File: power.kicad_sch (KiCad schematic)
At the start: 23 parts, among them J11 Conn_01x02_Socket, Q1 IPD068P03L3, U17 CJ9340, U30 ADS1110, U31 LMR51420YDDCR

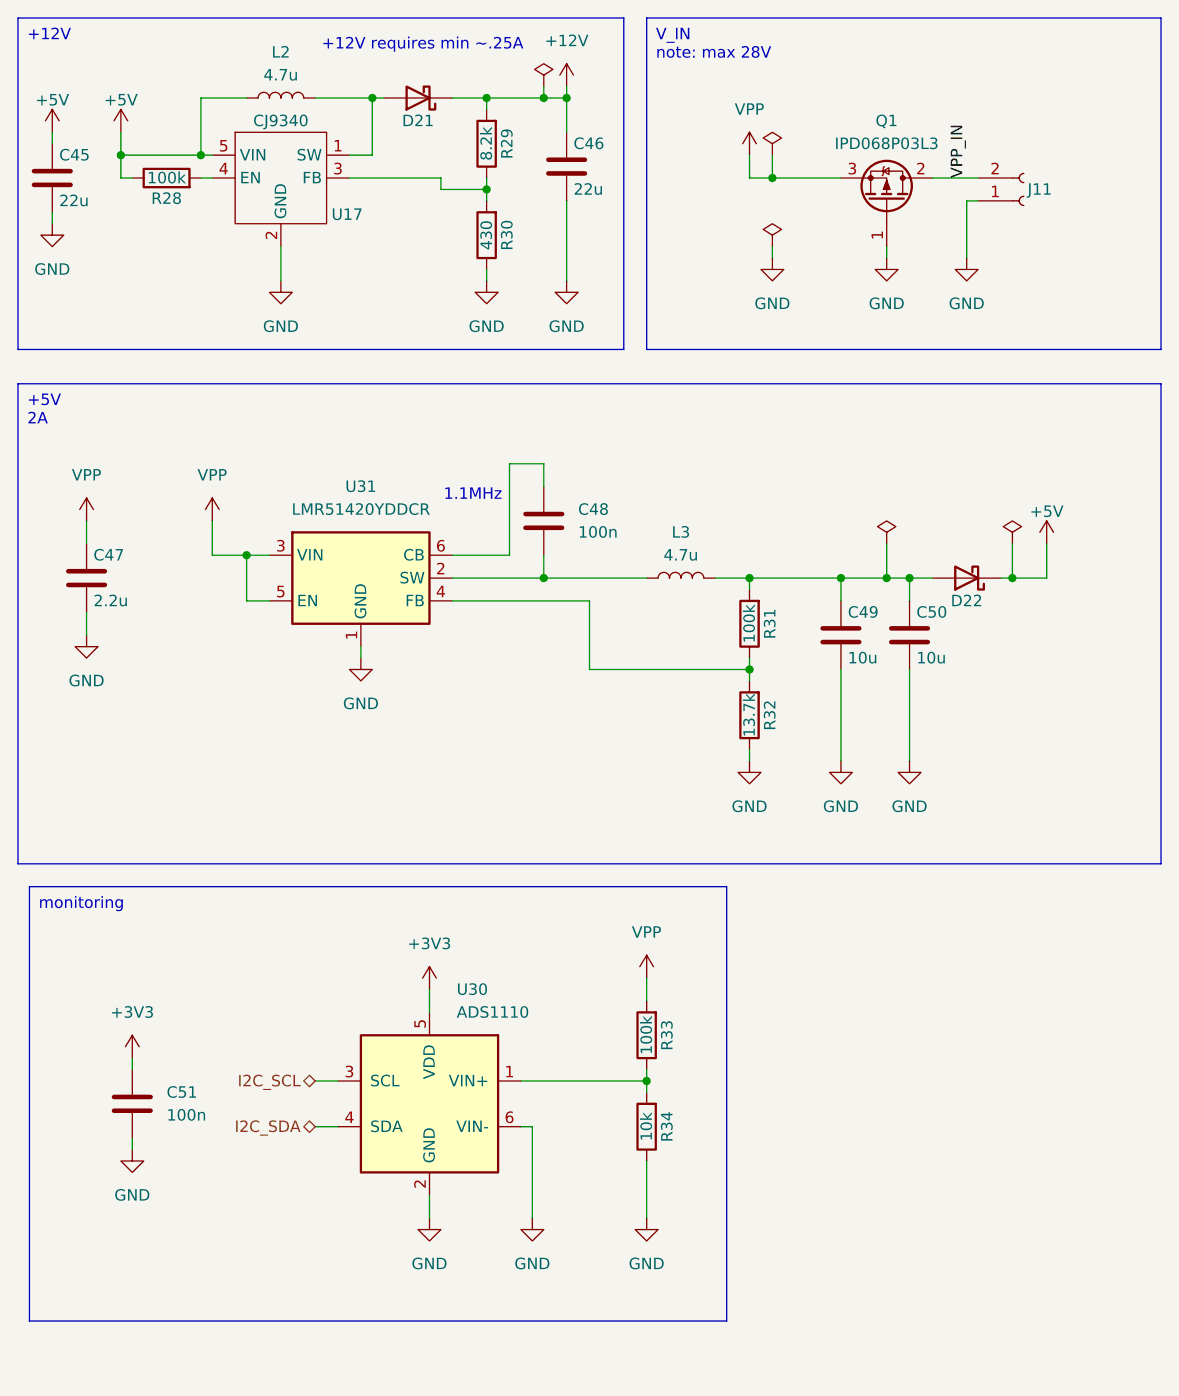
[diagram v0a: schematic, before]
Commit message: tiny last minute fixes
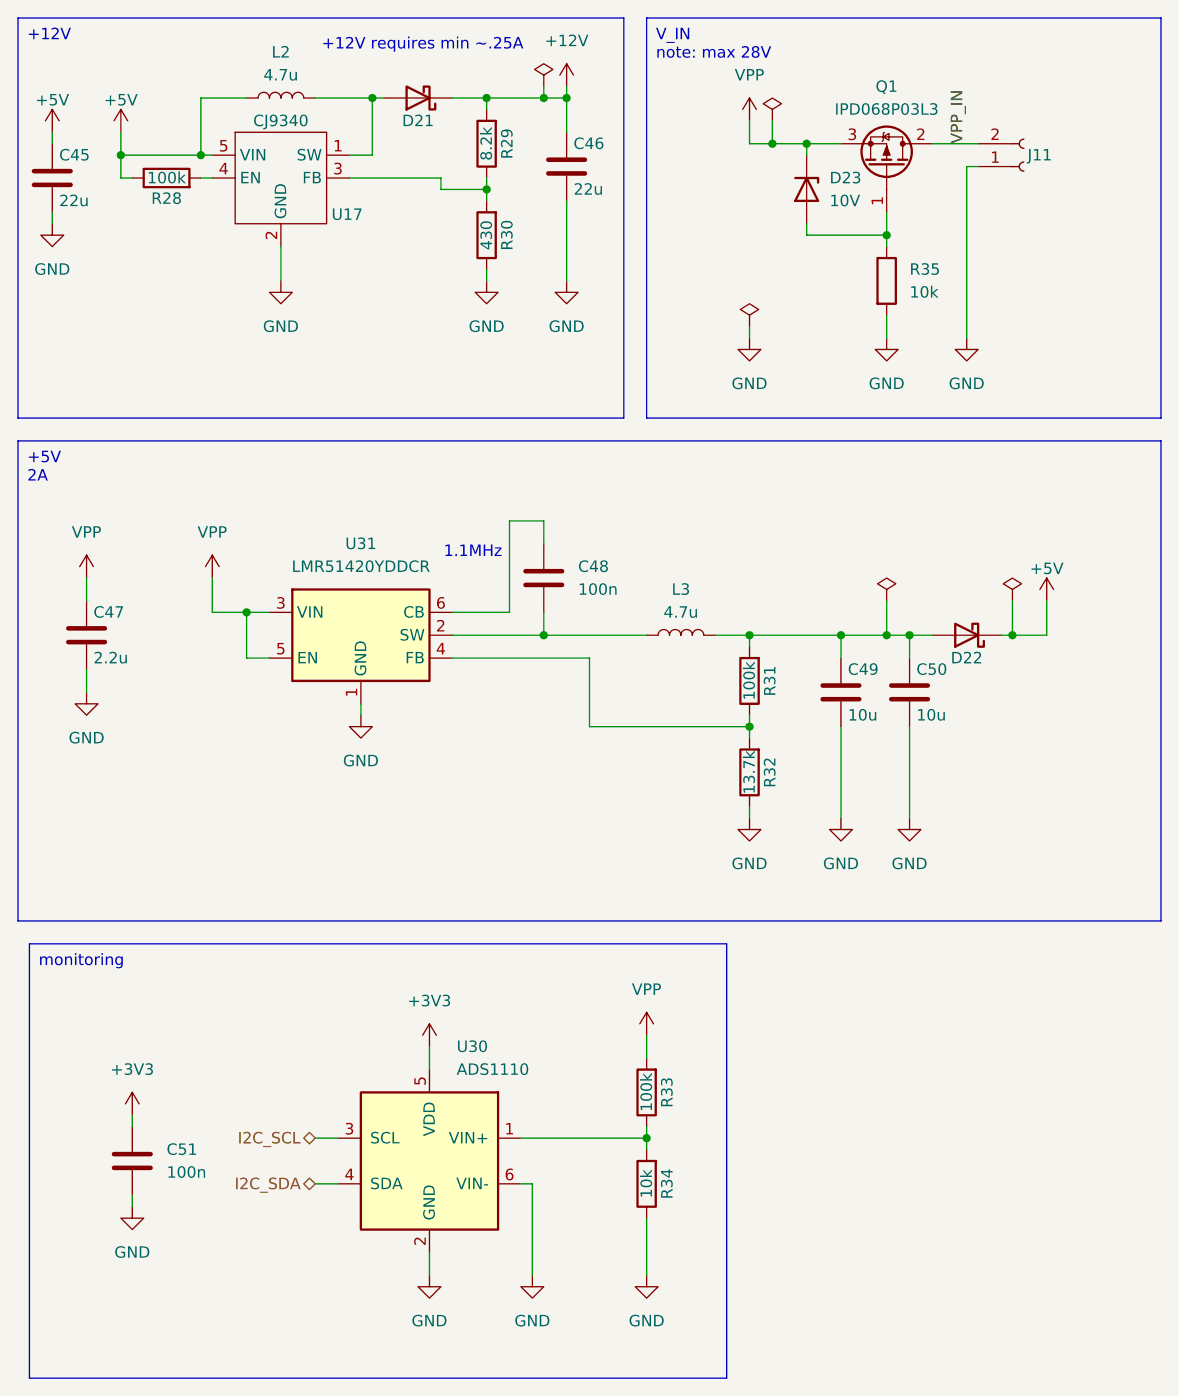
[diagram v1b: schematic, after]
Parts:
- added D23: 10V, Diode_SMD:D_SOD-323, symbol Device:D_Zener
- added R35: 10k, Resistor_SMD:R_0402_1005Metric, symbol Device:R
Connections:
- net GND: now also R35.2; no longer Q1.1 (G)
- net VPP: now also D23.1 (K)
- new net: D23.2 (A), Q1.1 (G), R35.1
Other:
- moved on the sheet: C47, C48, C49, C50, C51, D22, J11, L3, Q1, R31, R32, R33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
